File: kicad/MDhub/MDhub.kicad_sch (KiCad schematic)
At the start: 49 parts, among them J1 USB_C_Receptacle_USB2.0_14P, J10 Conn_01x04_Pin, J11 Conn_01x02_Pin, J12 Conn_01x04_Pin, J13 Conn_01x03_Pin, J14 Conn_01x03_Pin, J15 Conn_01x03_Pin, J16 Conn_01x03_Pin, J17 Conn_01x05_Pin, J18 Conn_01x05_Pin, J19 Conn_01x02_Pin, J2 Conn_01x04_Pin, J20 Conn_01x04_Pin, J3 Conn_01x05_Pin, J4 Conn_01x05_Pin, J5 Conn_01x05_Pin, J6 Conn_01x05_Pin, J7 Conn_01x02_Pin, J8 Conn_01x02_Pin, J9 Conn_01x04_Pin, SW1 SW_Wuerth_450301014042, U1 SOP-J8, U2 STM32H523CCTx, X1 IQXO-70

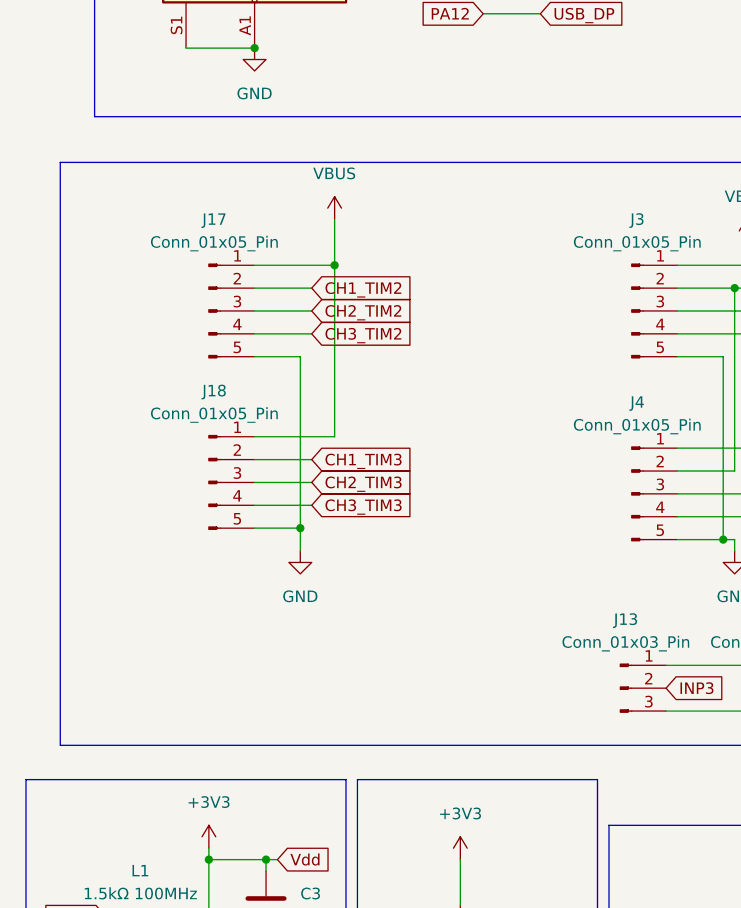
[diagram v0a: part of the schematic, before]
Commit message: perf MDhub circuit
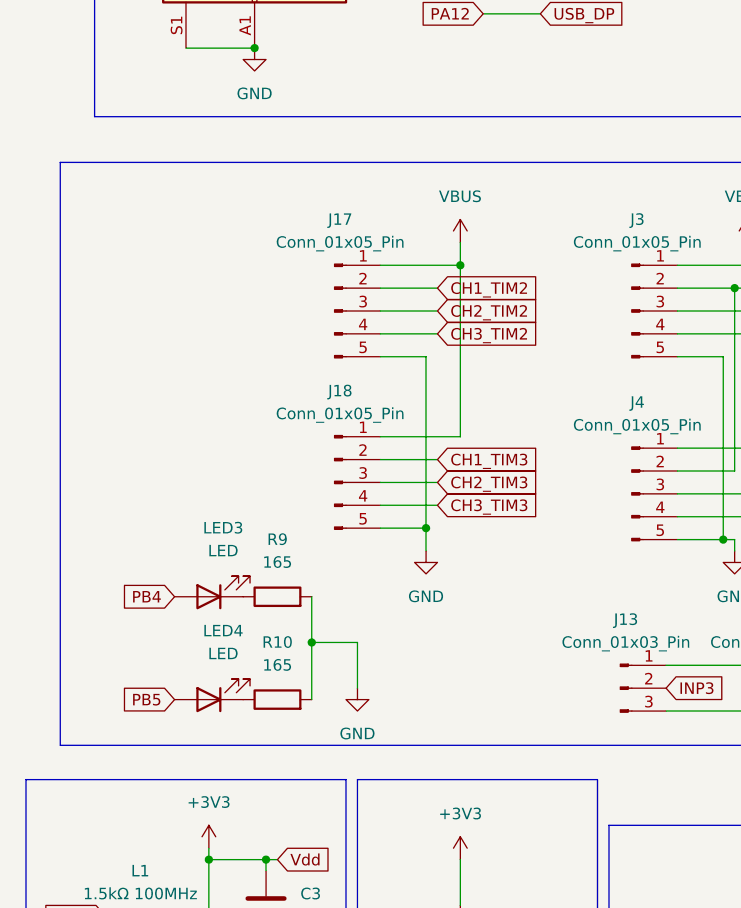
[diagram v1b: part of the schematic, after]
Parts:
- added LED3, LED4: LED, LED_SMD:LED_0603_1608Metric_Pad1.05x0.95mm_HandSolder, symbol Device:LED
- added R10, R9: 165, Resistor_SMD:R_0603_1608Metric_Pad0.98x0.95mm_HandSolder, symbol Device:R
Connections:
- net GND: now also R10.2, R9.2
- net PB4: now also LED3.2 (A)
- net PB5: now also LED4.2 (A)
- new net: LED4.1 (K), R10.1
- new net: LED3.1 (K), R9.1
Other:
- moved on the sheet: J17, J18

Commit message: finish
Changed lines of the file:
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@@
 (kicad_sch
-	(version 20231120)
+	(version 20250114)
 	(generator "eeschema")
-	(generator_version "8.0")
+	(generator_version "9.0")
 	(paper "A4")
